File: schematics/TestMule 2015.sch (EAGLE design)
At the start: 13 parts, among them K1 CB1A-P-12V, K2 CB1A-P-12V

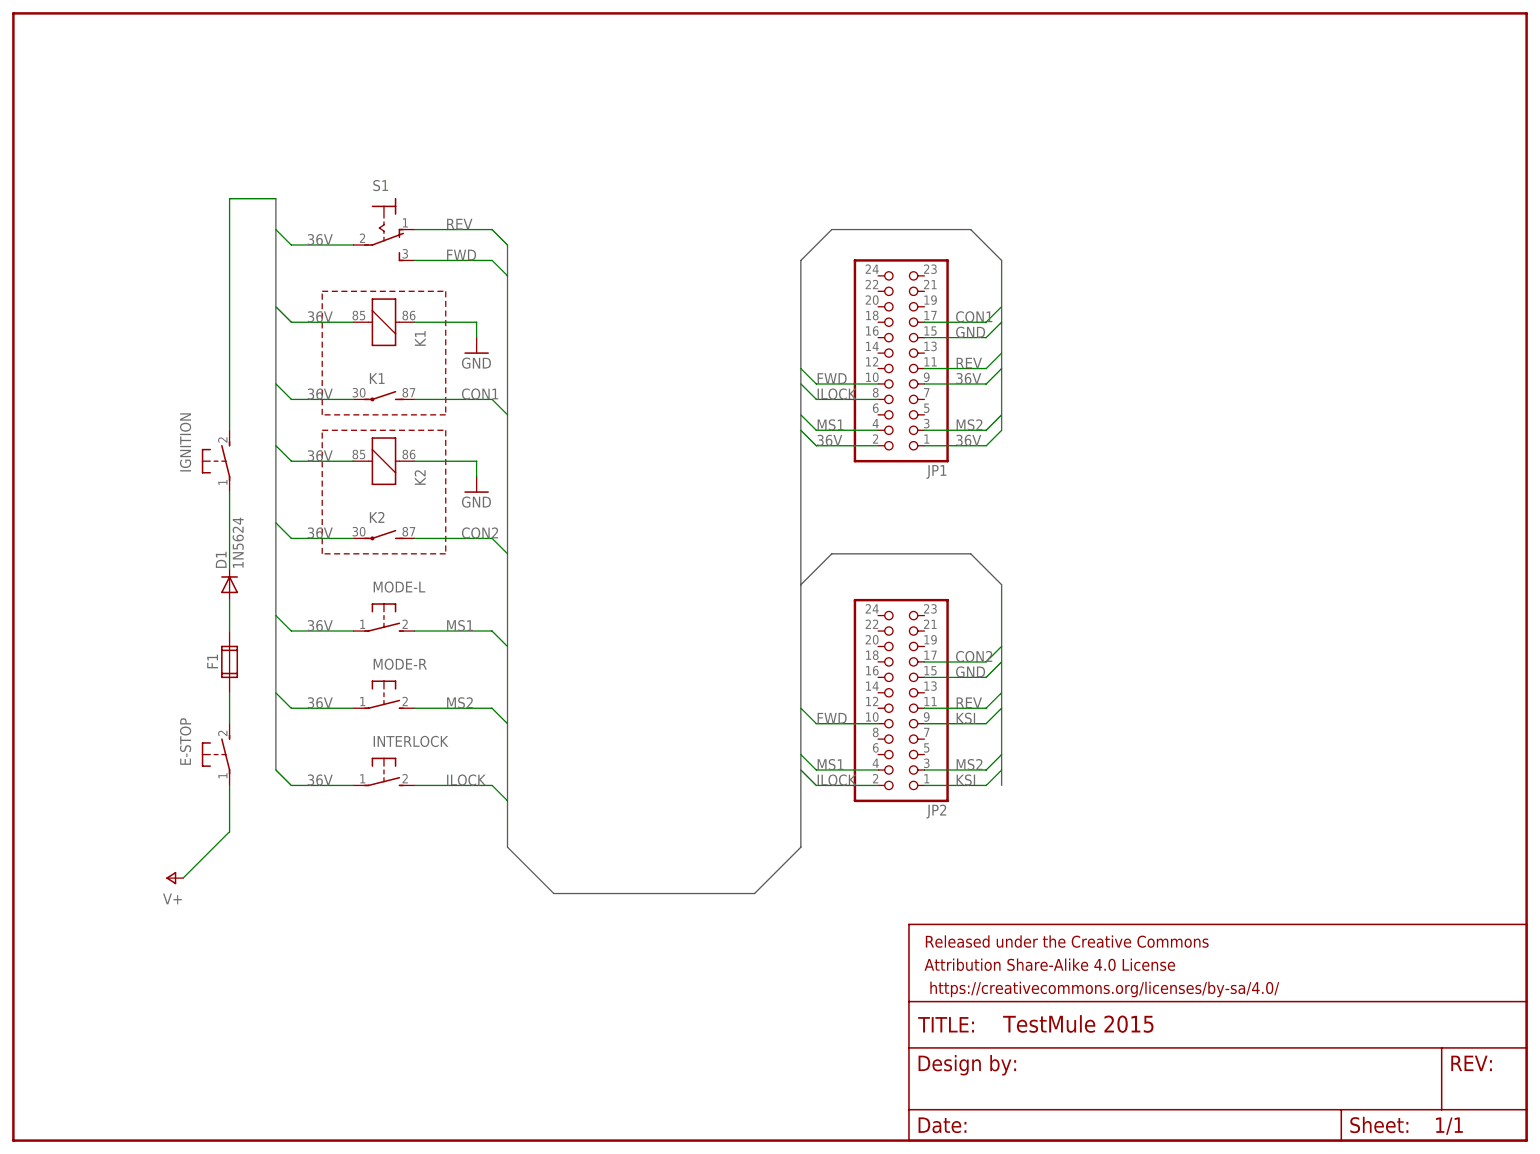
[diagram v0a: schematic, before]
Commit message: Debug defines
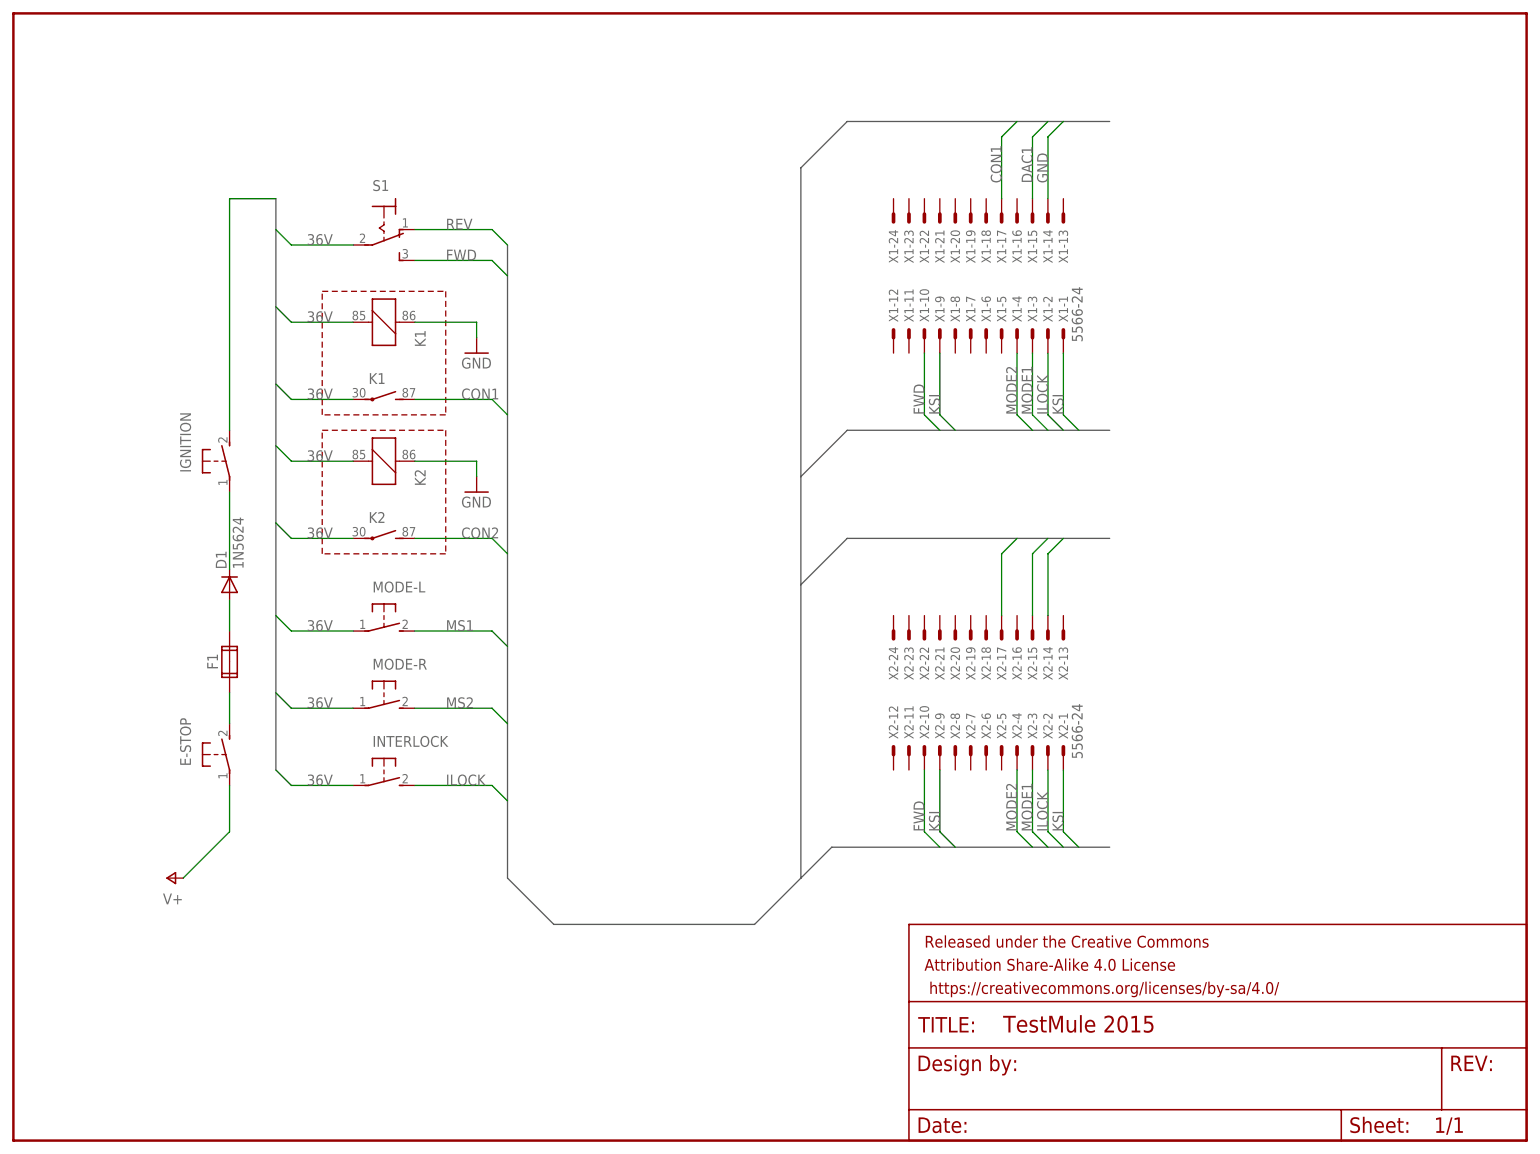
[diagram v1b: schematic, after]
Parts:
- removed JP1, JP2: (no value), pinhead:PINHD-2X12
- added X1, X2: 5566-24, con-molex:5566-24
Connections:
- new net DAC1: X1-15.S
- new net DAC2: X2-15.S
- new net MODE1: X1-3.S, X2-3.S
- new net MODE2: X1-4.S, X2-4.S
- net 36V: no longer JP1.1, JP1.2, JP1.9
- net CON1: now also X1-17.S, X2-17.S; no longer JP1.17
- net CON2: no longer JP2.17
- net FWD: now also X1-10.S, X2-10.S; no longer JP1.10, JP2.10
- net GND: now also X1-14.S, X2-14.S; no longer JP1.15, JP2.15
- net ILOCK: now also X1-2.S, X2-2.S; no longer JP1.8, JP2.2
- net KSI: now also X1-1.S, X1-9.S, X2-1.S, X2-9.S; no longer JP2.1, JP2.9
- net MS1: no longer JP1.4, JP2.4
- net MS2: no longer JP1.3, JP2.3
- net REV: no longer JP1.11, JP2.11
